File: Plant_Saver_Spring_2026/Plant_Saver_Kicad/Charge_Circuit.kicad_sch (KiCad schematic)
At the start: 22 parts, among them J1 1.25mm, Q1 G09P02L, Q12 G09P02L, Q2 G09P02L, Q3 G09P02L, Q4 ISP12DP06NMXTSA1, Q5 G09P02L, Q8 G09P02L, Q9 G09P02L, SW6 SA72SB0, U10 DW03C, U15 CDBA140SL-HF

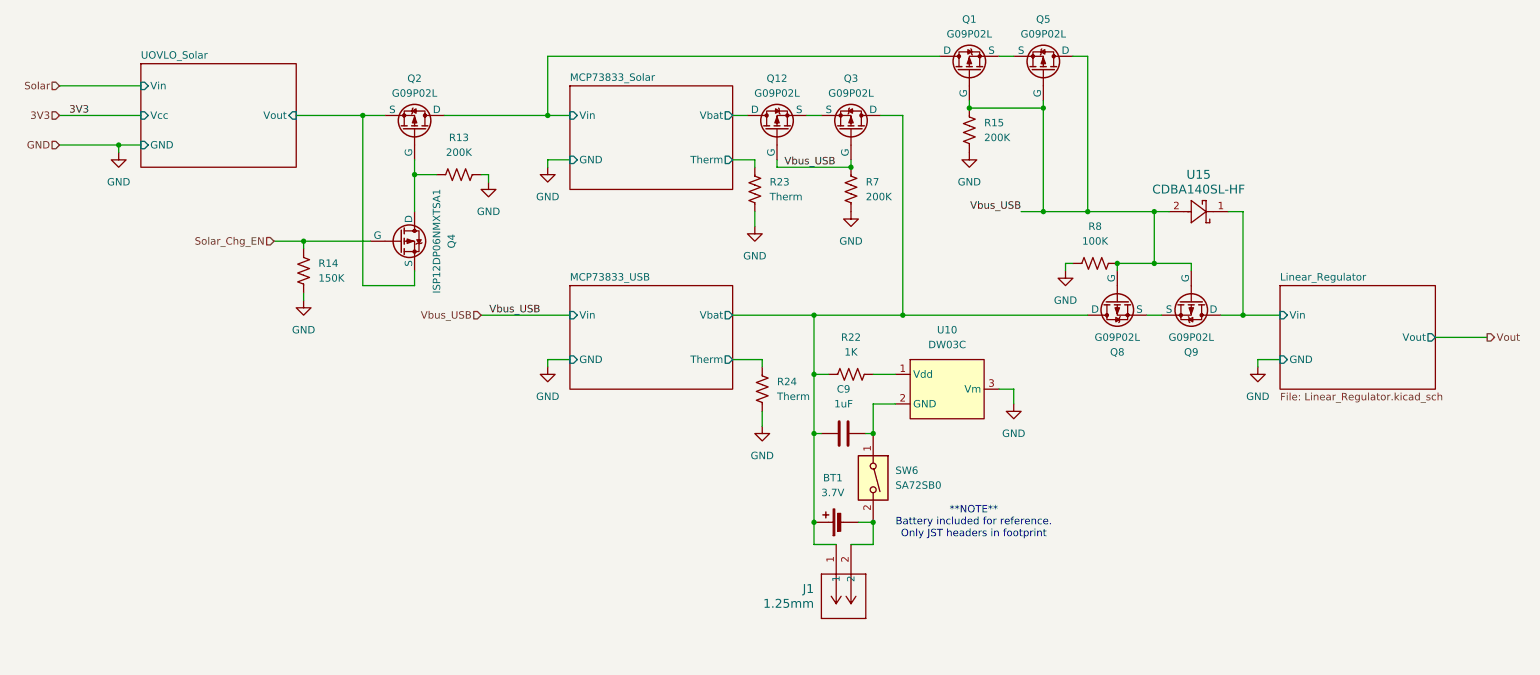
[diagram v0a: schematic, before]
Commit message: Minor updates to charge/power
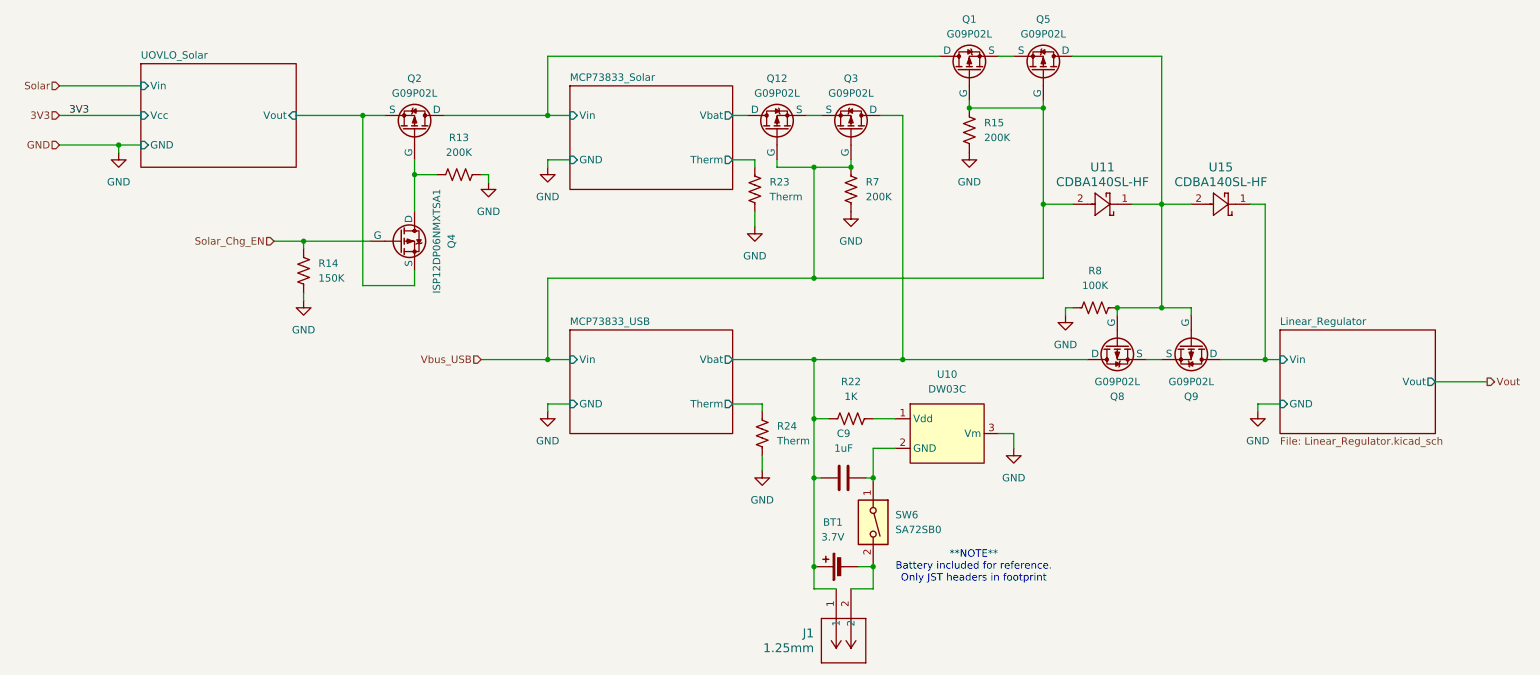
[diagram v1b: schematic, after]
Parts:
- added U11: CDBA140SL-HF, CDBA-HF, symbol CDBA140SL_HF:CDBA140SL-HF
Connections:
- net Vbus_USB: now also U11.2; no longer Q5.1 (D), Q8.2 (G), Q9.2 (G), R8.1, U15.2
- new net: Q5.1 (D), Q8.2 (G), Q9.2 (G), R8.1, U11.1, U15.2
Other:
- moved on the sheet: BT1, C9, J1, Q8, Q9, R22, R24, R8, SW6, U10, U15
